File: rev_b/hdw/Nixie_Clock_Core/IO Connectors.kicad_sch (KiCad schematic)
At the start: 0 parts

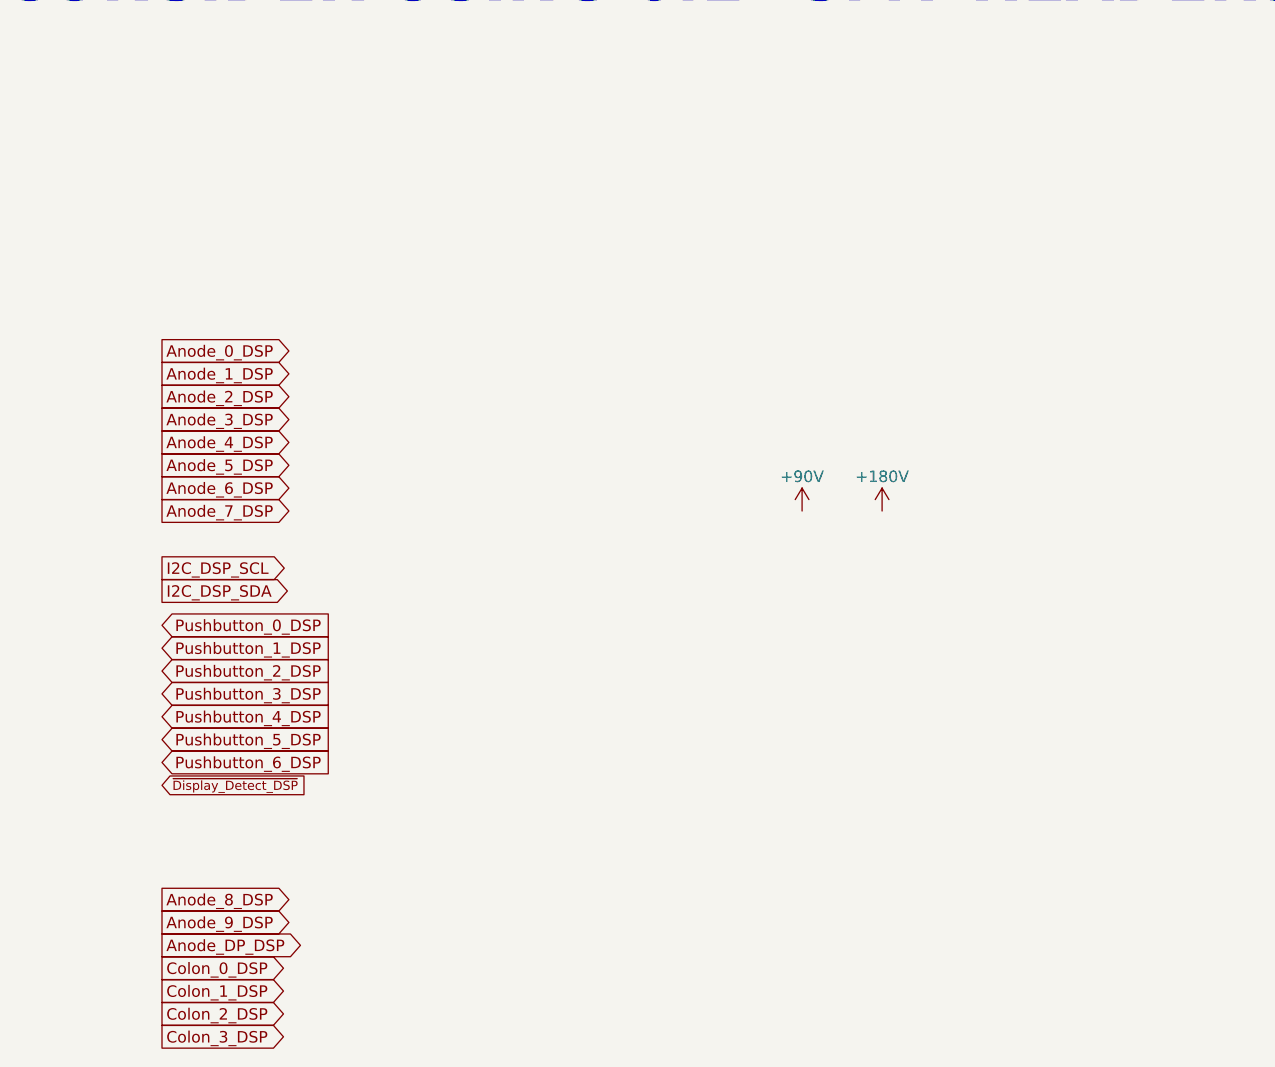
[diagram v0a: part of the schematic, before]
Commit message: more carrier board progress
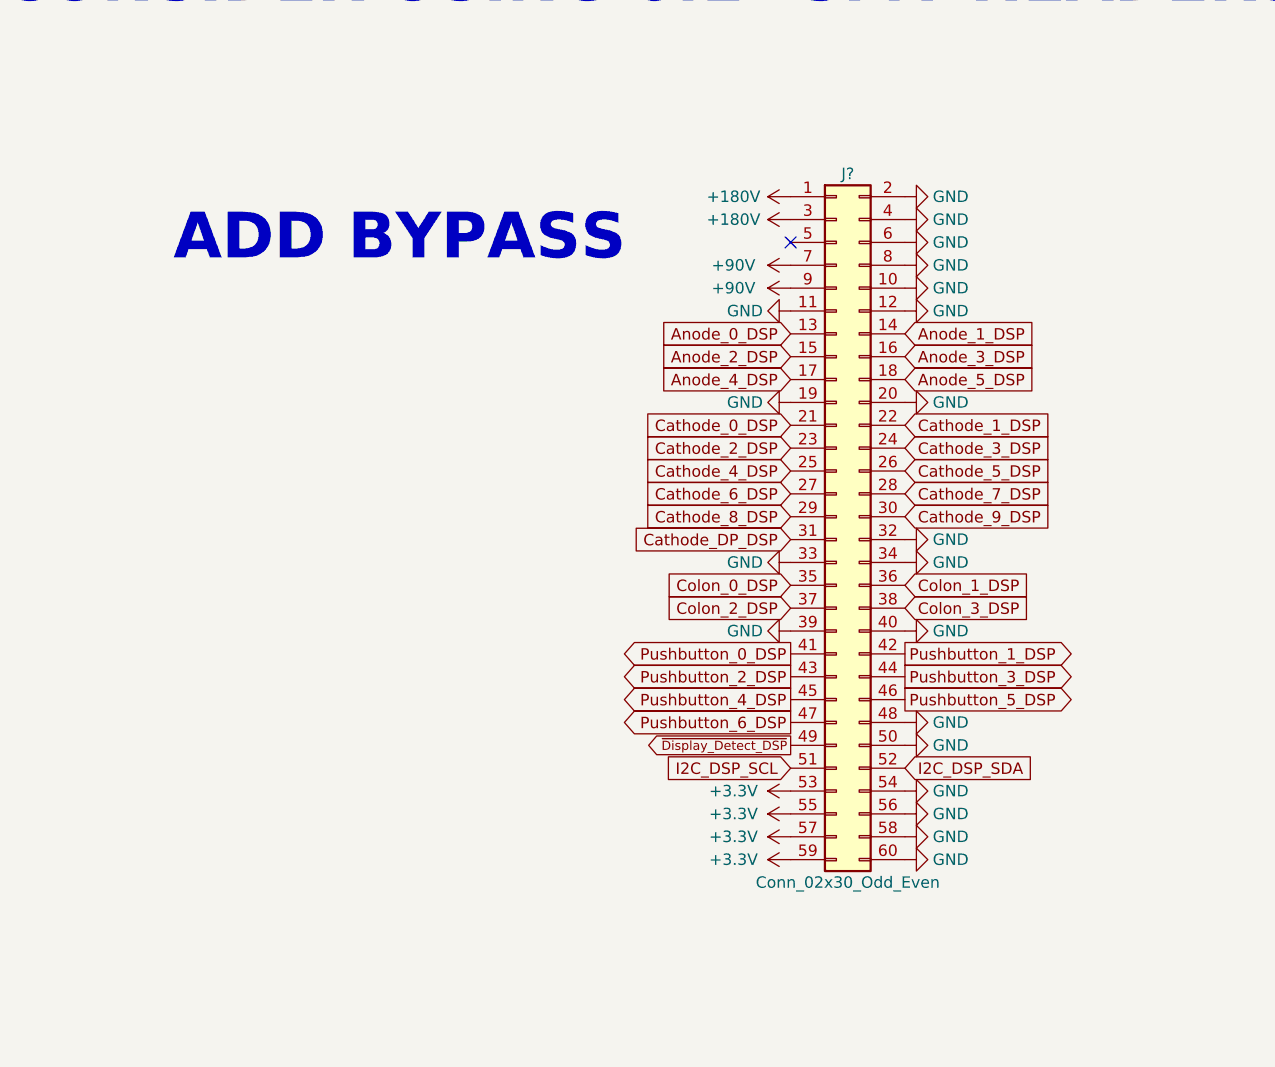
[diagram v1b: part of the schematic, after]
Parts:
- added J?: Conn_02x30_Odd_Even, symbol Connector_Generic:Conn_02x30_Odd_Even
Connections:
- net +180V: now also J?.1 (Pin_1), J?.3 (Pin_3), J?.7 (Pin_7), J?.9 (Pin_9)
- net Anode_0_DSP: now also J?.13 (Pin_13)
- net Anode_1_DSP: now also J?.14 (Pin_14)
- net Anode_2_DSP: now also J?.15 (Pin_15)
- net Anode_3_DSP: now also J?.16 (Pin_16)
- net Anode_4_DSP: now also J?.17 (Pin_17)
- net Anode_5_DSP: now also J?.18 (Pin_18)
- net Colon_0_DSP: now also J?.35 (Pin_35)
- net Colon_1_DSP: now also J?.36 (Pin_36)
- net Colon_2_DSP: now also J?.37 (Pin_37)
- net Colon_3_DSP: now also J?.38 (Pin_38)
- net I2C_DSP_SCL: now also J?.51 (Pin_51)
- net I2C_DSP_SDA: now also J?.52 (Pin_52)
- net Pushbutton_0_DSP: now also J?.41 (Pin_41)
- net Pushbutton_1_DSP: now also J?.42 (Pin_42)
- net Pushbutton_2_DSP: now also J?.43 (Pin_43)
- net Pushbutton_3_DSP: now also J?.44 (Pin_44)
- net Pushbutton_4_DSP: now also J?.45 (Pin_45)
- net Pushbutton_5_DSP: now also J?.46 (Pin_46)
- net Pushbutton_6_DSP: now also J?.47 (Pin_47)
- net ~{Display_Detect_DSP}: now also J?.49 (Pin_49)
- new net +3.3V: J?.53 (Pin_53), J?.55 (Pin_55), J?.57 (Pin_57), J?.59 (Pin_59)
- new net Cathode_0_DSP: J?.21 (Pin_21)
- new net Cathode_1_DSP: J?.22 (Pin_22)
- new net Cathode_2_DSP: J?.23 (Pin_23)
- new net Cathode_3_DSP: J?.24 (Pin_24)
- new net Cathode_4_DSP: J?.25 (Pin_25)
- new net Cathode_5_DSP: J?.26 (Pin_26)
- new net Cathode_6_DSP: J?.27 (Pin_27)
- new net Cathode_7_DSP: J?.28 (Pin_28)
- new net Cathode_8_DSP: J?.29 (Pin_29)
- new net Cathode_9_DSP: J?.30 (Pin_30)
- new net Cathode_DP_DSP: J?.31 (Pin_31)
- new net GND: J?.10 (Pin_10), J?.11 (Pin_11), J?.12 (Pin_12), J?.19 (Pin_19), J?.2 (Pin_2), J?.20 (Pin_20), J?.32 (Pin_32), J?.33 (Pin_33), J?.34 (Pin_34), J?.39 (Pin_39), J?.4 (Pin_4), J?.40 (Pin_40), J?.48 (Pin_48), J?.50 (Pin_50), J?.54 (Pin_54), J?.56 (Pin_56), J?.58 (Pin_58), J?.6 (Pin_6), J?.60 (Pin_60), J?.8 (Pin_8)
- no-connect marks 0 -> 1
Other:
- note added: "ADD BYPASS"
